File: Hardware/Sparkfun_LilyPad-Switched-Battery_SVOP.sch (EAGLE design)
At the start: 13 parts

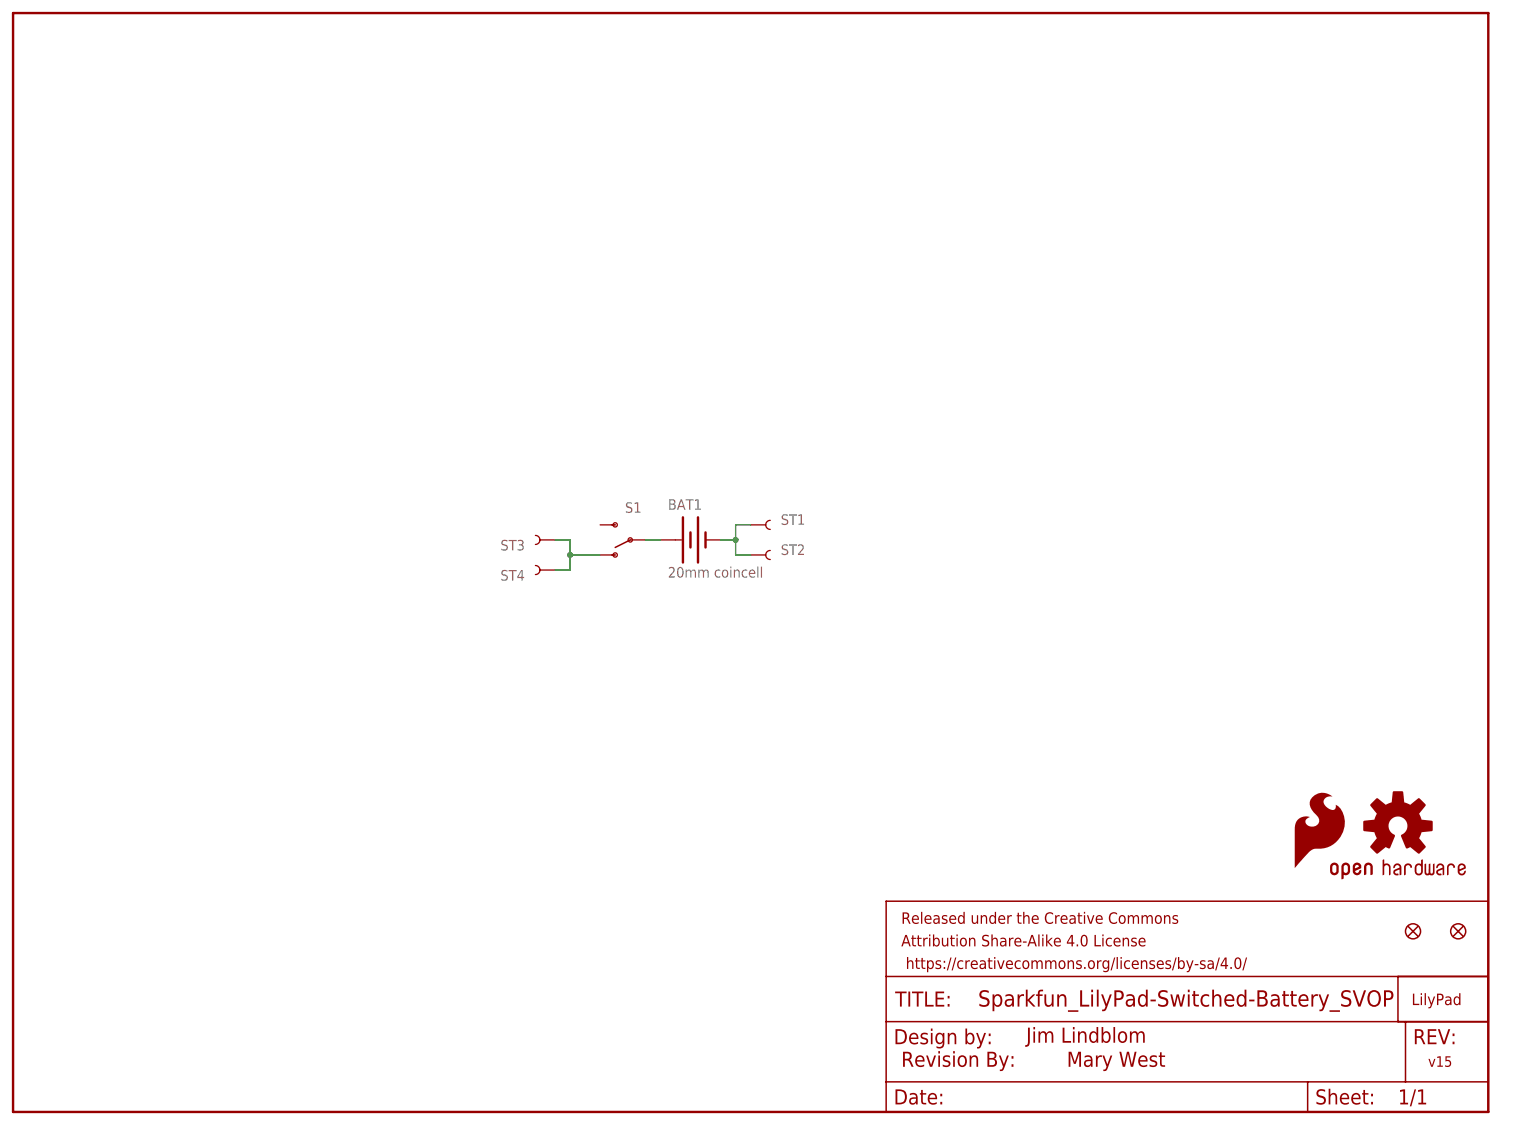
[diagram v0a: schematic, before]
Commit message: Cleaning up Repo
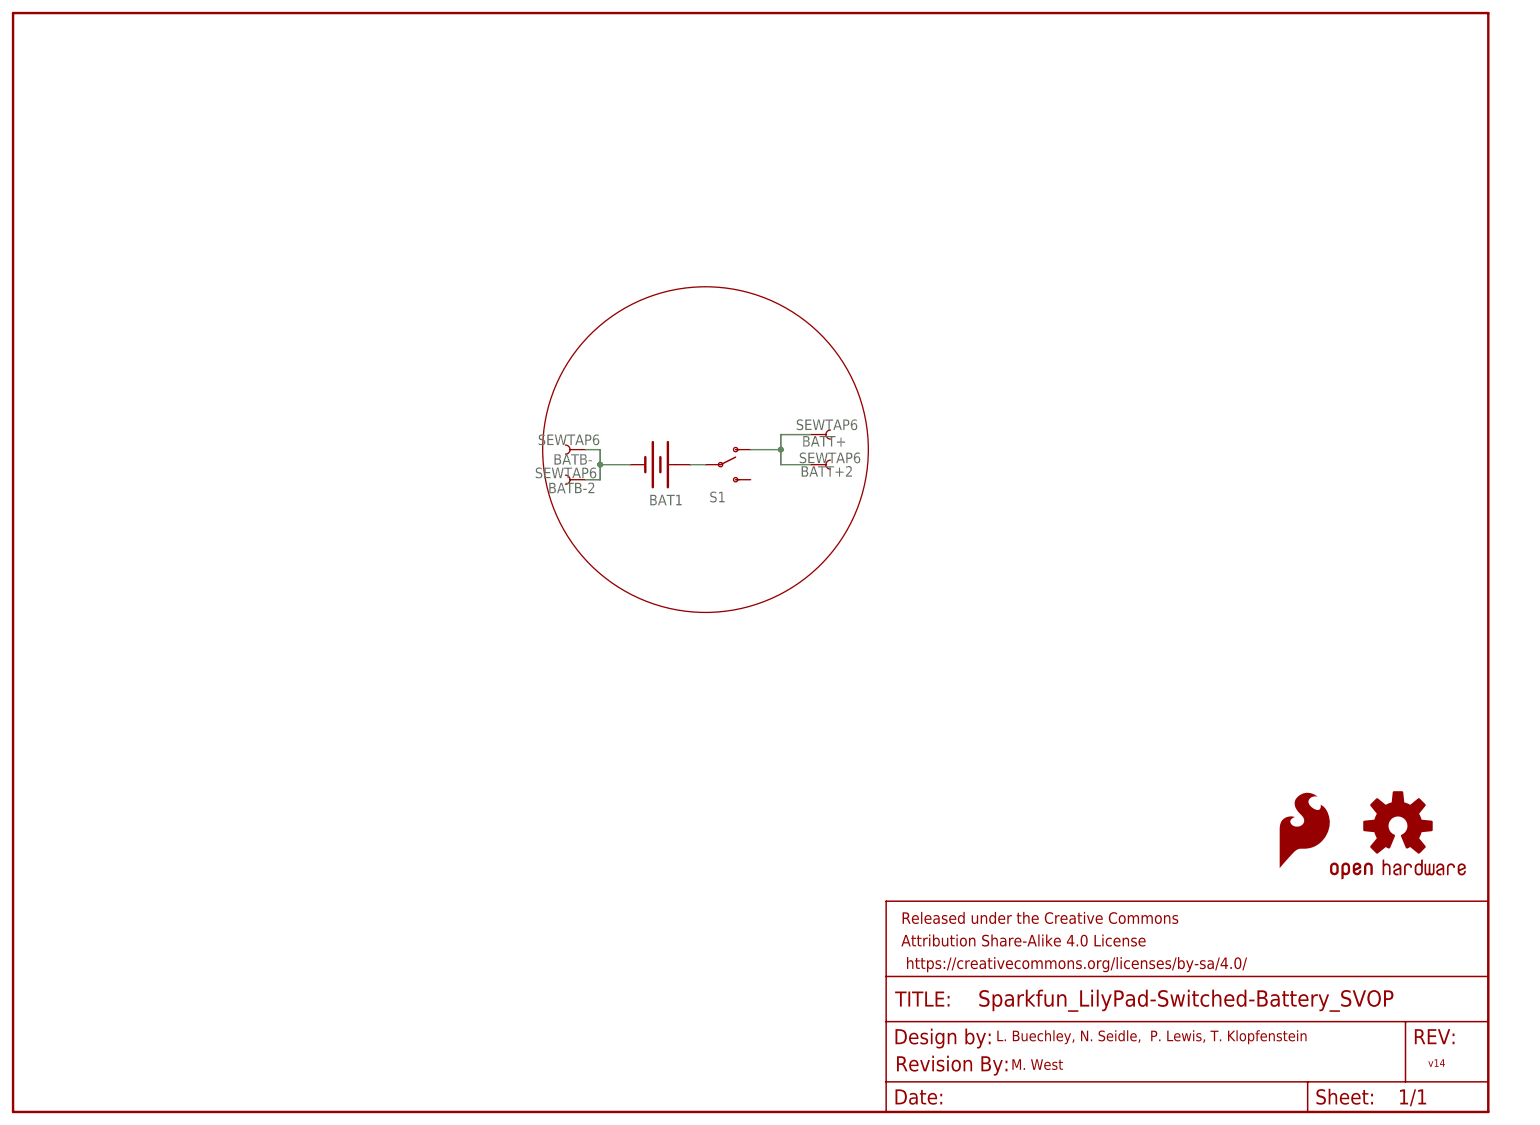
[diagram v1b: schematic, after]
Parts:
- removed JP1, JP2: FIDUCIALUFIDUCIAL, SparkFun-Aesthetics:FIDUCIALUFIDUCIAL
- removed ST1, ST2, ST3, ST4: SEWTAP6, LilyPad-Wearables:SEWTAP6
- removed U$5: LOGO-LPLP, LilyPad-Wearables:LOGO-LPLP
- added BATB-, BATB-2, BATT+, BATT+2: SEWTAP6, LilyPad-Wearables:SEWTAP6
- renumbered U$7 to LOGO2
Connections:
- removed net N$1 (its old number): S1.O, ST3.1, ST4.1
- new net GND: BAT1.-, BATB-.1, BATB-2.1
- net N$2: now also BATT+.1, BATT+2.1, S1.O; no longer BAT1.-, ST1.1, ST2.1
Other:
- note added: "L. Buechley, N. Seidle, P. Lewis, T. Klopfenstein"
- note added: "M. West"
- note added: "v14"
- note removed: "Jim Lindblom"
- note removed: "Mary West"
- note removed: "v15"
- moved on the sheet: BAT1, S1
